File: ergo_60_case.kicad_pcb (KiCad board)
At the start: 2 copper layers, 285 x 94.6 mm, 163 parts, among them SW1 SW_Push, U1 PRTR5V0U2X, U2 OLED_SSD1306, U3 AT90USB1286-AU, U4 AVR-ISP, Y1 16MHz

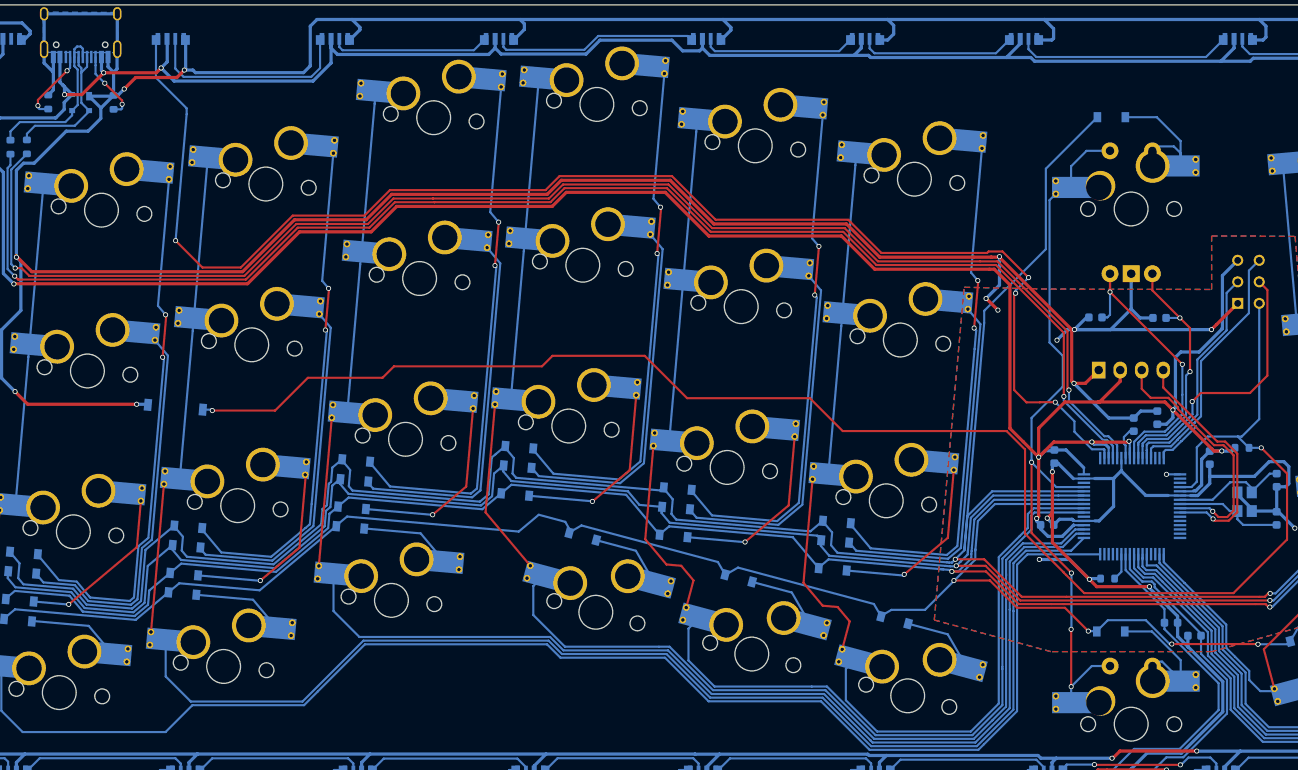
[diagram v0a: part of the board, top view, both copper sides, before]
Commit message: updates for prod
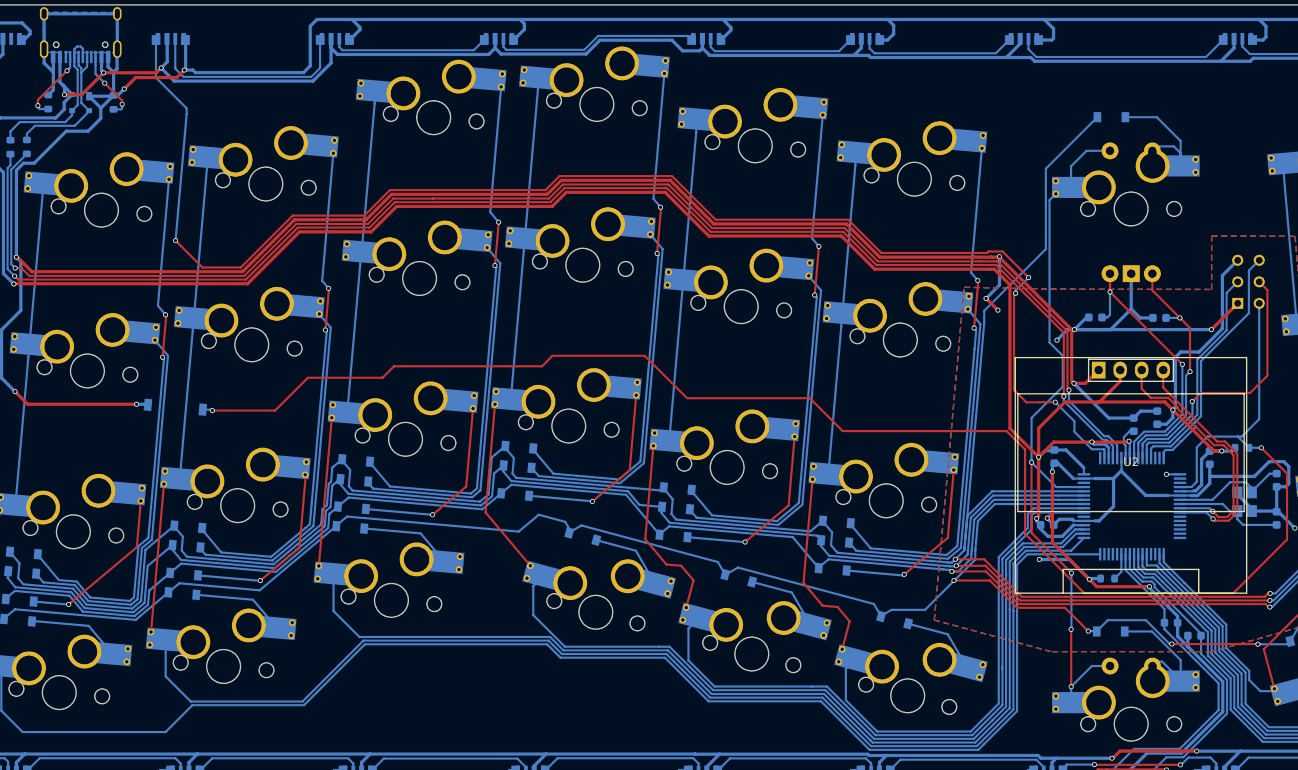
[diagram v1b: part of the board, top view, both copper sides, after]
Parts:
- U2: footprint KiCadLibs:SSD1306_128x64OLED_wHoles -> KiCadLibs:SSD1306_128x64OLED
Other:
- rule pad_to_mask_clearance: 0 -> 0.05
